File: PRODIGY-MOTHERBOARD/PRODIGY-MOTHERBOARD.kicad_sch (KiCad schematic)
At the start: 0 parts

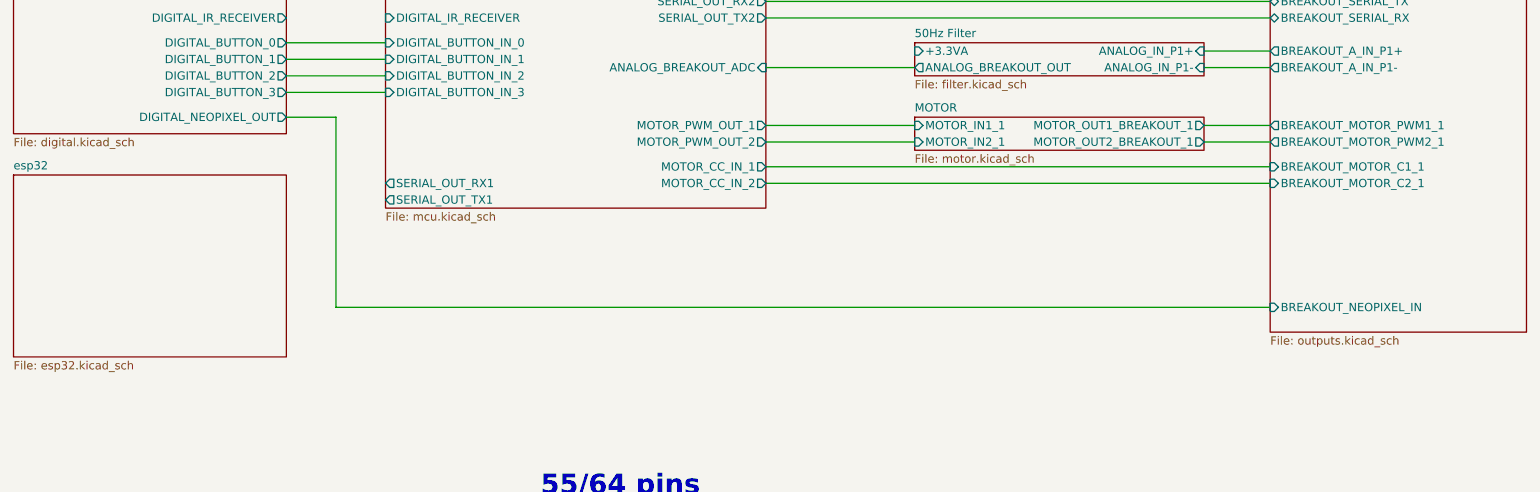
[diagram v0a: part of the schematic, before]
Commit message: Esp32 motherboard schematic done.
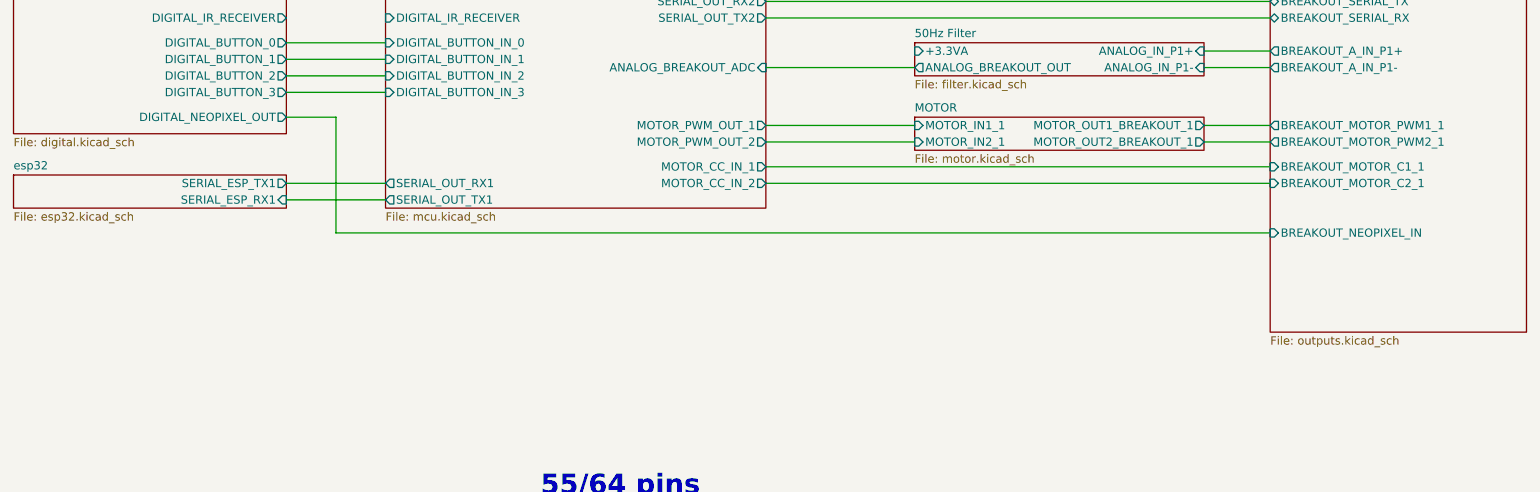
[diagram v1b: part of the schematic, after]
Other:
- sheet esp32 ports: added SERIAL_ESP_RX1, SERIAL_ESP_TX1; removed none
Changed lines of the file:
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@@
 	(wire
 		(pts
-			(xy 86.36 127) (xy 86.36 156.21)
+			(xy 78.74 139.7) (xy 93.98 139.7)
+		)
+		(stroke
+			(width 0)
+			(type default)
+		)
+	)
+	(wire
+		(pts
+			(xy 86.36 127) (xy 86.36 144.78)
 		)
 		(stroke
@@
 	(wire
 		(pts
-			(xy 86.36 156.21) (xy 229.87 156.21)
+			(xy 86.36 144.78) (xy 229.87 144.78)
 		)
 		(stroke
@@
 		(pts
 			(xy 78.74 127) (xy 86.36 127)
+		)
+		(stroke
+			(width 0)
+			(type default)
+		)
+	)
+	(wire
+		(pts
+			(xy 78.74 137.16) (xy 93.98 137.16)
 		)
 		(stroke
@@
 	(sheet
 		(at 36.83 135.89)
-		(size 41.91 27.94)
+		(size 41.91 5.08)
 		(fields_autoplaced yes)
 		(stroke
@@
 		)
 		(property "Sheetfile" "esp32.kicad_sch"
-			(at 36.83 164.4146 0)
+			(at 36.83 141.5546 0)
 			(effects
 				(font
@@
 				)
 				(hide yes)
+			)
+		)
+		(pin "SERIAL_ESP_RX1" input
+			(at 78.74 139.7 0)
+			(effects
+				(font
+					(size 1.27 1.27)
+				)
+				(justify right)
+			)
+		)
+		(pin "SERIAL_ESP_TX1" output
+			(at 78.74 137.16 0)
+			(effects
+				(font
+					(size 1.27 1.27)
+				)
+				(justify right)
 			)
 		)
@@
 		)
 		(pin "BREAKOUT_NEOPIXEL_IN" input
-			(at 229.87 156.21 180)
-			(effects
-				(font
+			(at 229.87 144.78 180)
+			(effects
+				(font
